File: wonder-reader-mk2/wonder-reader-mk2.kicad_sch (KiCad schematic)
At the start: 20 parts, among them J1 Conn_01x04_Pin, J2 Conn_01x02_Pin, J4 Conn_01x02_Pin, J5 Conn_01x08_Pin, J6 Conn_01x04_Pin, J7 Conn_01x10_MountingPin, U1 ESP32-DevKitC, U2 A4988_STEPPER_MOTOR_DRIVER_CA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, U3 AMS1117-3.3, U5 74HC595, U6 MAX98357A

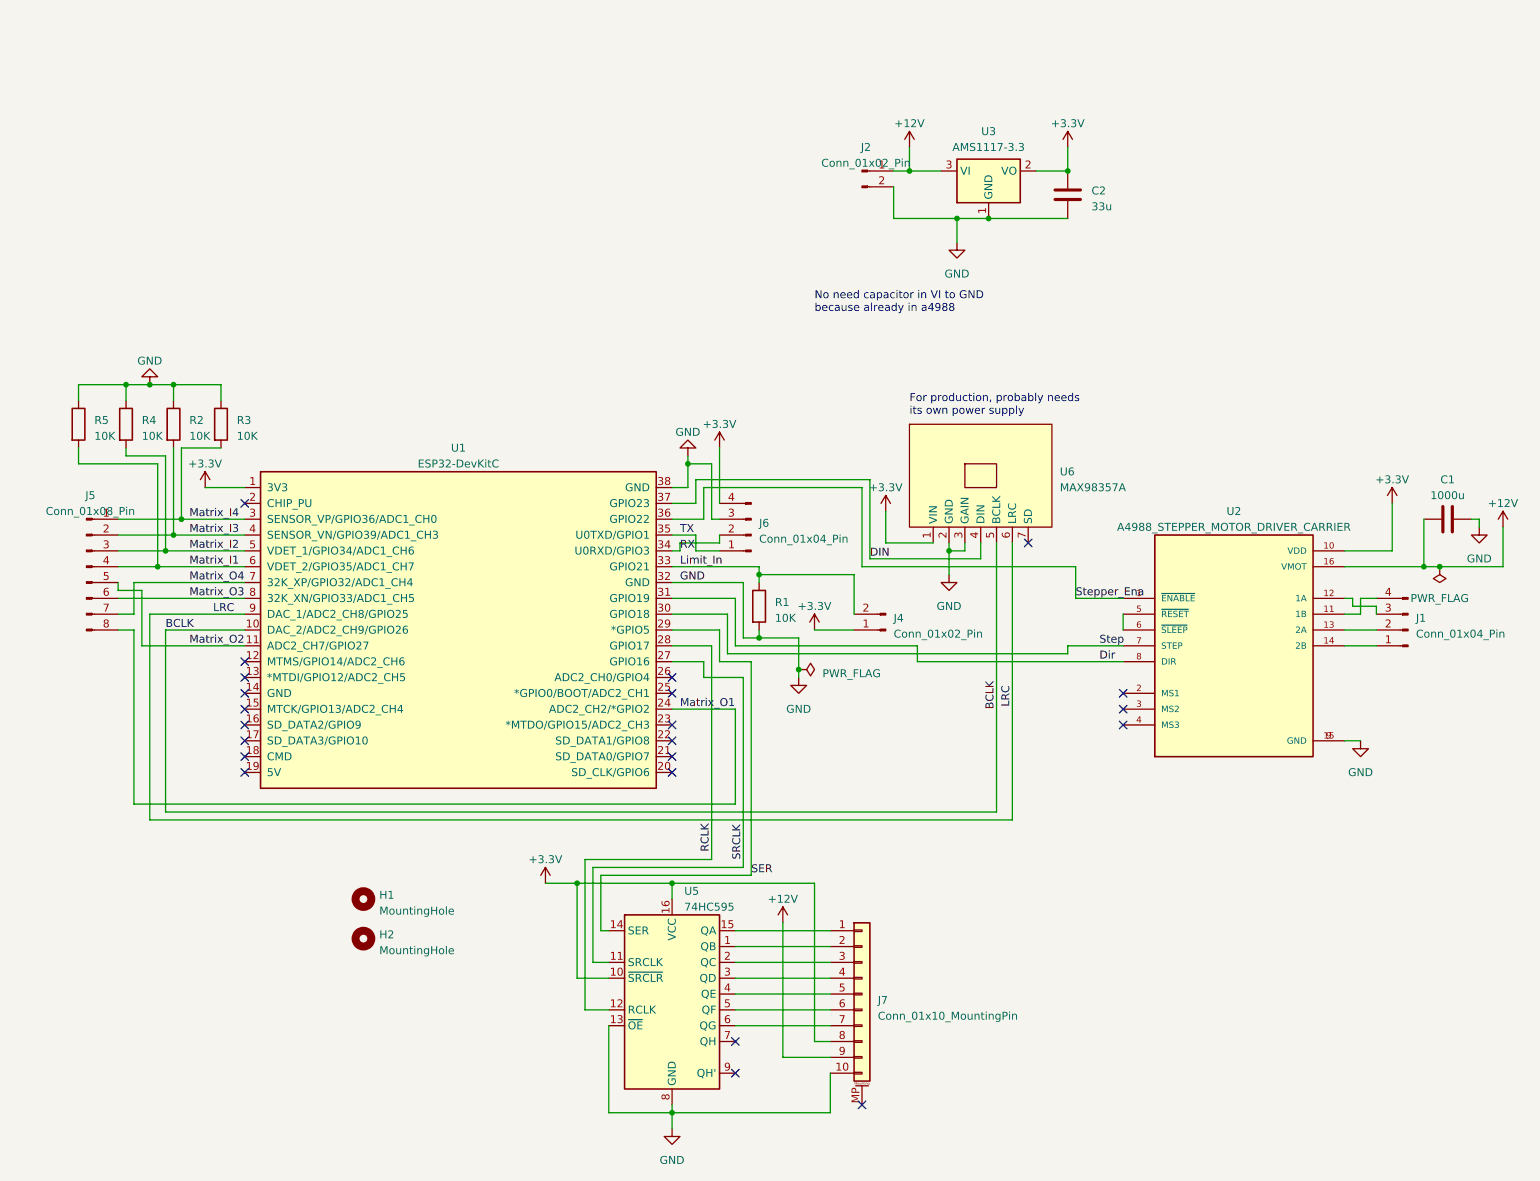
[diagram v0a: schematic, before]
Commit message: PCB and new models for mark 2
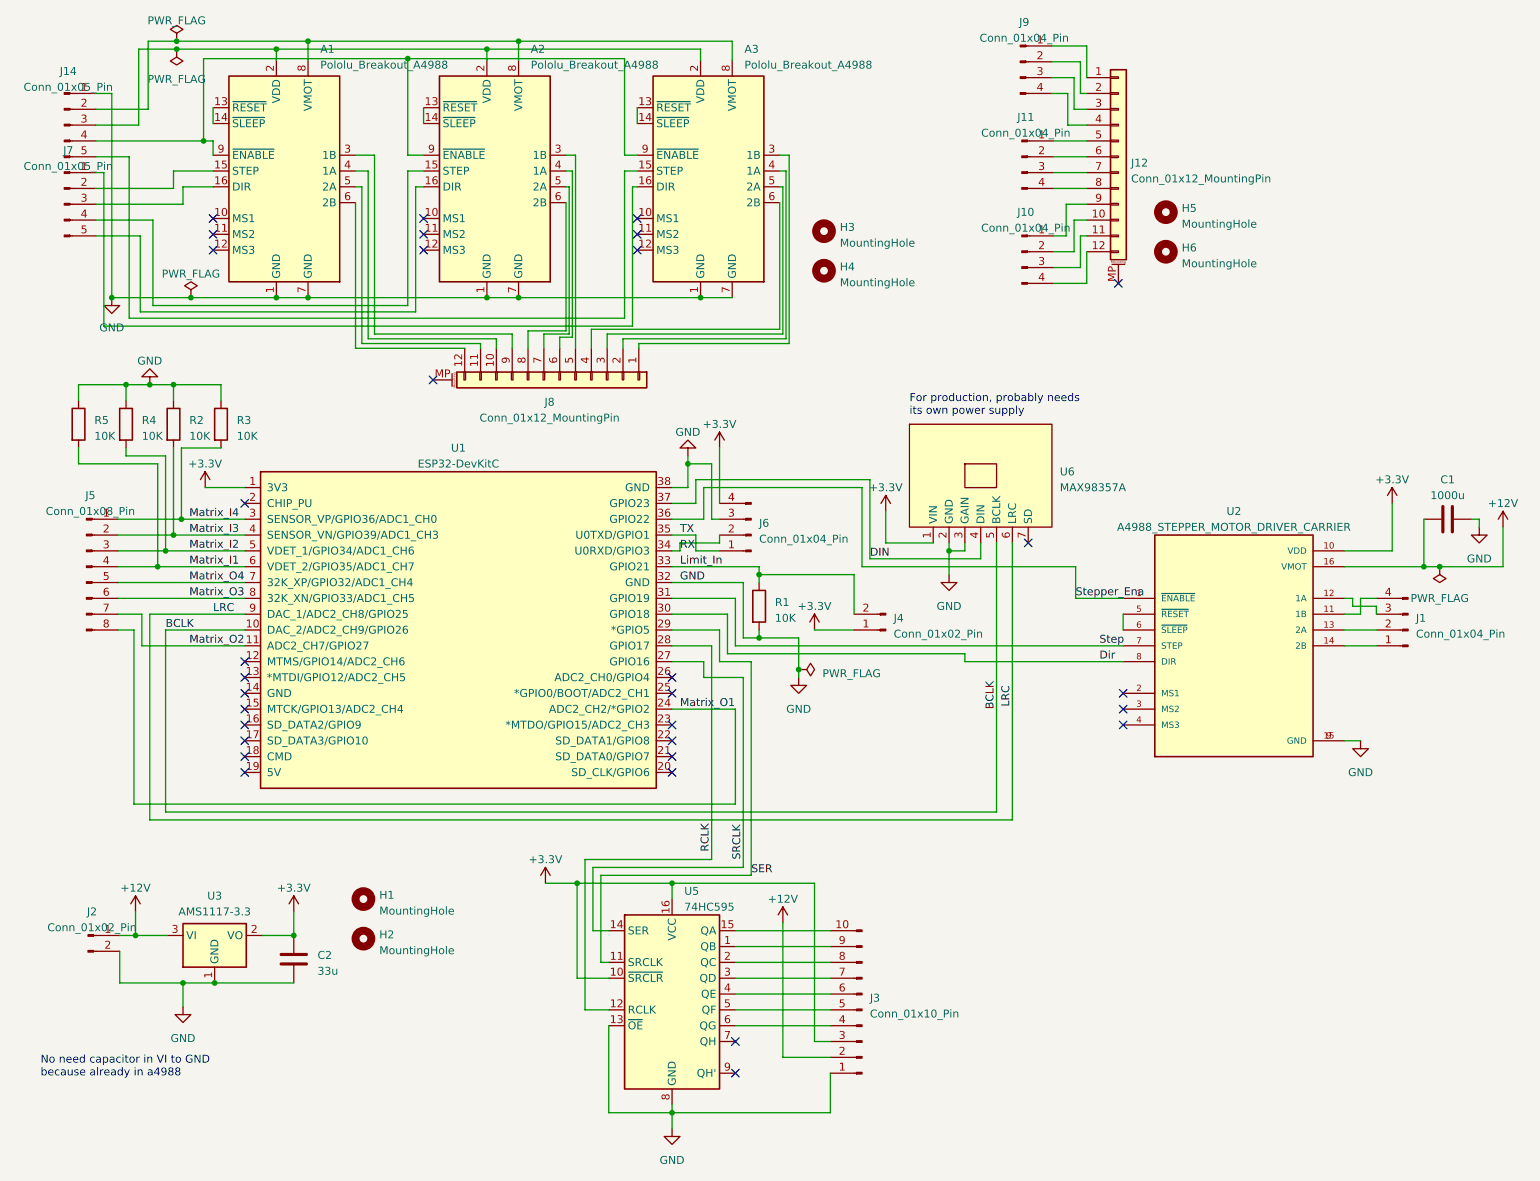
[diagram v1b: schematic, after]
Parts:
- removed J7: Conn_01x10_MountingPin, Connector_FFC-FPC:Hirose_FH12-10S-0.5SH_1x10-1MP_P0.50mm_Horizontal, symbol Connector_Generic_MountingPin:Conn_01x10_MountingPin
- added A1, A2, A3: Pololu_Breakout_A4988, Module:Pololu_Breakout-16_15.2x20.3mm, symbol Driver_Motor:Pololu_Breakout_A4988
- added H3, H4, H5, H6: MountingHole, MountingHole:MountingHole_2.2mm_M2, symbol Mechanical:MountingHole
- added J10, J11, J9: Conn_01x04_Pin, Connector_PinHeader_2.54mm:PinHeader_1x04_P2.54mm_Vertical, symbol Connector:Conn_01x04_Pin
- added J12, J8: Conn_01x12_MountingPin, Connector_FFC-FPC:Hirose_FH12-12S-0.5SH_1x12-1MP_P0.50mm_Horizontal, symbol Connector_Generic_MountingPin:Conn_01x12_MountingPin
- added J14, J7: Conn_01x05_Pin, Connector_PinHeader_2.54mm:PinHeader_1x05_P2.54mm_Vertical, symbol Connector:Conn_01x05_Pin
- added J3: Conn_01x10_Pin, Connector_PinHeader_2.54mm:PinHeader_1x10_P2.54mm_Vertical, symbol Connector:Conn_01x10_Pin
- J1: footprint Connector_PinSocket_2.54mm:PinSocket_1x04_P2.54mm_Vertical -> Connector_PinHeader_2.54mm:PinHeader_1x04_P2.54mm_Vertical
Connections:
- net +12V: now also J3.2 (Pin_2)
- net +3.3V: now also J3.3 (Pin_3)
- net Dir: now also U1.30 (GPIO18); no longer U1.31 (GPIO19)
- net GND: now also A1.1 (GND), A1.7 (GND), A2.1 (GND), A2.7 (GND), A3.1 (GND), A3.7 (GND), J14.1 (Pin_1), J3.1 (Pin_1)
- net Matrix_O2: now also J5.7 (Pin_7); no longer J5.5 (Pin_5)
- net Matrix_O4: now also J5.5 (Pin_5); no longer J5.7 (Pin_7)
- net SER: now also U5.11 (SRCLK); no longer U5.14 (SER)
- net SRCLK: now also U5.14 (SER); no longer U5.11 (SRCLK)
- net Step: now also U1.31 (GPIO19); no longer U1.30 (GPIO18)
- net at U5.15 (QA): now also J3.10 (Pin_10)
- net at U5.1 (QB): now also J3.9 (Pin_9)
- net at U5.2 (QC): now also J3.8 (Pin_8)
- net at U5.3 (QD): now also J3.7 (Pin_7)
- net at U5.4 (QE): now also J3.6 (Pin_6)
- net at U5.5 (QF): now also J3.5 (Pin_5)
- net at U5.6 (QG): now also J3.4 (Pin_4)
- new net: J12.1 (Pin_1), J9.1 (Pin_1)
- new net: J10.2 (Pin_2), J12.10 (Pin_10)
- new net: J10.3 (Pin_3), J12.11 (Pin_11)
- new net: J10.4 (Pin_4), J12.12 (Pin_12)
- new net: J12.2 (Pin_2), J9.2 (Pin_2)
- new net: J12.3 (Pin_3), J9.3 (Pin_3)
- new net: J12.4 (Pin_4), J9.4 (Pin_4)
- new net: J11.1 (Pin_1), J12.5 (Pin_5)
- new net: J11.2 (Pin_2), J12.6 (Pin_6)
- new net: J11.3 (Pin_3), J12.7 (Pin_7)
- new net: J11.4 (Pin_4), J12.8 (Pin_8)
- new net: J10.1 (Pin_1), J12.9 (Pin_9)
- new net: A1.8 (VMOT), A2.8 (VMOT), A3.8 (VMOT), J14.2 (Pin_2)
- new net: A1.2 (VDD), A2.2 (VDD), A3.2 (VDD), J14.3 (Pin_3)
- new net: A1.9 (~{ENABLE}), A2.9 (~{ENABLE}), A3.9 (~{ENABLE}), J14.4 (Pin_4)
- new net: A3.15 (STEP), J14.5 (Pin_5)
- new net: A3.13 (~{RESET}), A3.14 (~{SLEEP})
- new net: A3.16 (DIR), J7.1 (Pin_1)
- new net: A3.3 (1B), J8.1 (Pin_1)
- new net: A3.4 (1A), J8.2 (Pin_2)
- new net: A3.5 (2A), J8.3 (Pin_3)
- new net: A3.6 (2B), J8.4 (Pin_4)
- new net: A1.4 (1A), J8.10 (Pin_10)
- new net: A1.5 (2A), J8.11 (Pin_11)
- new net: A1.6 (2B), J8.12 (Pin_12)
- new net: A2.3 (1B), J8.5 (Pin_5)
- new net: A2.4 (1A), J8.6 (Pin_6)
- new net: A2.5 (2A), J8.7 (Pin_7)
- new net: A2.6 (2B), J8.8 (Pin_8)
- new net: A1.3 (1B), J8.9 (Pin_9)
- new net: A1.15 (STEP), J7.2 (Pin_2)
- new net: A1.16 (DIR), J7.3 (Pin_3)
- new net: A2.15 (STEP), J7.4 (Pin_4)
- new net: A2.16 (DIR), J7.5 (Pin_5)
- new net: A1.13 (~{RESET}), A1.14 (~{SLEEP})
- new net: A2.13 (~{RESET}), A2.14 (~{SLEEP})
- no-connect marks 22 -> 32
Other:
- moved on the sheet: C2, J2, U3
